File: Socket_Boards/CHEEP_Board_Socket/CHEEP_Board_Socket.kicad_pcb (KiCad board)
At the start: 4 copper layers, 64.9 x 71.4 mm, 70 parts

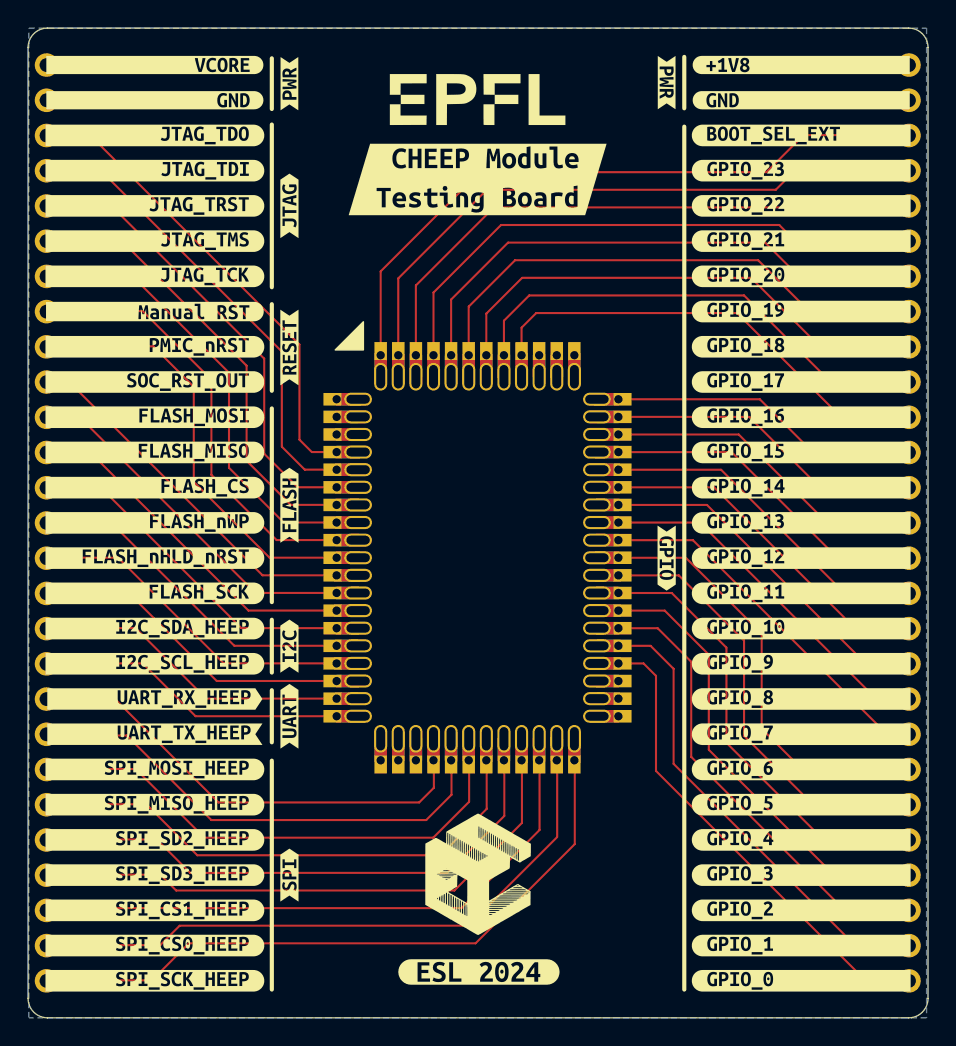
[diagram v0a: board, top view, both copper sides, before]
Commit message: Big push. Fixed the issues that were pending. See github
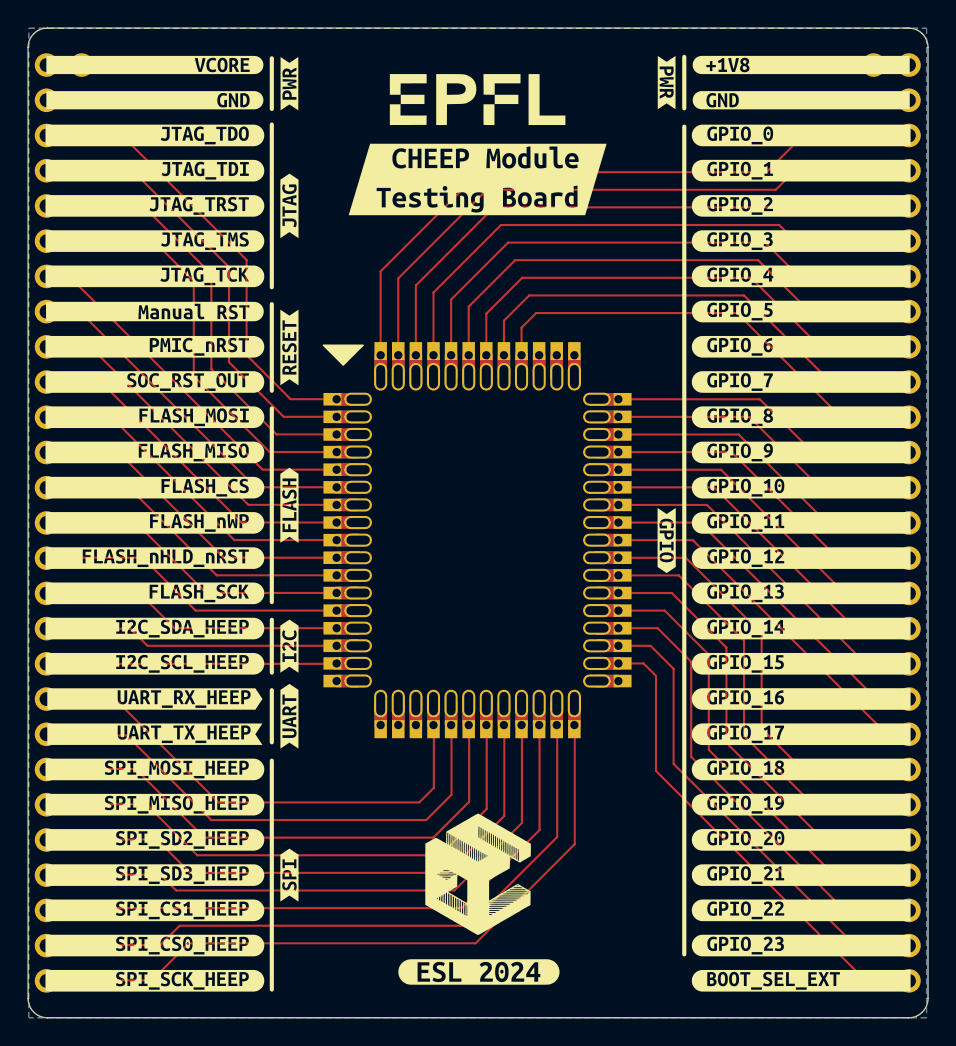
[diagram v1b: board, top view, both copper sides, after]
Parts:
- moved kibuzzard-66E70DDA 61.0 mm to (165.7, 135.3)
- moved kibuzzard-66E70EAB 61.0 mm to (165.7, 74.3)
- moved kibuzzard-66E70E24 55.9 mm to (165.7, 132.7)
- moved kibuzzard-66E70EA7 55.9 mm to (165.7, 76.8)
- moved kibuzzard-66E70E1C 50.8 mm to (165.7, 130.2)
- moved kibuzzard-66E70E9D 50.8 mm to (165.7, 79.4)
- moved kibuzzard-66E70E2E 45.7 mm to (165.7, 127.6)
- moved kibuzzard-66E70E98 45.7 mm to (165.7, 81.9)
- moved kibuzzard-66E70E32 40.6 mm to (165.7, 125.1)
- moved kibuzzard-66E70E93 40.6 mm to (165.7, 84.5)
- moved kibuzzard-66E70E38 35.6 mm to (165.7, 122.6)
- moved kibuzzard-66E70E8D 35.6 mm to (165.7, 87.0)
- moved kibuzzard-66E70E42 30.5 mm to (165.7, 120.0)
- moved kibuzzard-66E70E85 30.5 mm to (165.7, 89.5)
- moved kibuzzard-66E70E46 25.4 mm to (165.7, 117.5)
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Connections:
- J1 pad 1: VCORE -> Net-(J1A-JTAG_TDO)
- J1 pad 10: Net-(J1A-PMIC_nRST) -> Net-(J1A-FLASH_MISO)
- J1 pad 11: Net-(J1A-SOC_RST_OUT) -> Net-(J1A-FLASH_CS)
- J1 pad 12: Net-(J1A-FLASH_MOSI) -> Net-(J1A-FLASH_nWP)
- J1 pad 13: Net-(J1A-FLASH_MISO) -> Net-(J1A-FLASH_nHLD_nRST)
- J1 pad 14: Net-(J1A-FLASH_CS) -> Net-(J1A-FLASH_SCK)
- J1 pad 15: Net-(J1A-FLASH_nWP) -> Net-(J1A-I2C_SDA_HEEP)
- J1 pad 16: Net-(J1A-FLASH_nHLD_nRST) -> Net-(J1A-I2C_SCL_HEEP)
- J1 pad 17: Net-(J1A-FLASH_SCK) -> GND
- J1 pad 18: Net-(J1A-I2C_SDA_HEEP) -> +1V8
- J1 pad 19: Net-(J1A-I2C_SCL_HEEP) -> VCORE
- J1 pad 2: +1V8 -> Net-(J1A-JTAG_TDI)
- J1 pad 20: +1V8 -> GND
- J1 pad 21: VCORE -> Net-(J1B-UART_RX_HEEP)
- J1 pad 22: GND -> Net-(J1B-UART_TX_HEEP)
- J1 pad 23: Net-(J1B-UART_RX_HEEP) -> Net-(J1B-SPI_MOSI_HEEP)
- J1 pad 24: Net-(J1B-UART_TX_HEEP) -> Net-(J1B-SPI_MISO_HEEP)
- J1 pad 25: Net-(J1B-SPI_MOSI_HEEP) -> Net-(J1B-SPI_SD2_HEEP)
- J1 pad 26: Net-(J1B-SPI_MISO_HEEP) -> Net-(J1B-SPI_SD3_HEEP)
- J1 pad 27: Net-(J1B-SPI_SD2_HEEP) -> Net-(J1B-SPI_CS1_HEEP)
- J1 pad 28: Net-(J1B-SPI_SD3_HEEP) -> Net-(J1B-SPI_CS0_HEEP)
- J1 pad 29: Net-(J1B-SPI_CS1_HEEP) -> Net-(J1B-SPI_SCK_HEEP)
- J1 pad 3: GND -> Net-(J1A-JTAG_TRST)
- J1 pad 30: Net-(J1B-SPI_CS0_HEEP) -> GND
- J1 pad 31: Net-(J1B-SPI_SCK_HEEP) -> Net-(J1C-BOOT_SEL_EXT)
- J1 pad 32: +1V8 -> Net-(J1C-GPIO_23)
- J1 pad 33: VCORE -> Net-(J1C-GPIO_22)
- J1 pad 34: GND -> Net-(J1C-GPIO_21)
- J1 pad 35: Net-(J1C-BOOT_SEL_EXT) -> Net-(J1C-GPIO_20)
- J1 pad 36: Net-(J1C-GPIO_23) -> Net-(J1C-GPIO_19)
- J1 pad 37: Net-(J1C-GPIO_22) -> Net-(J1C-GPIO_18)
- J1 pad 38: Net-(J1C-GPIO_21) -> Net-(J1C-GPIO_17)
- J1 pad 39: Net-(J1C-GPIO_20) -> Net-(J1C-GPIO_16)
- J1 pad 4: Net-(J1A-JTAG_TDO) -> Net-(J1A-JTAG_TMS)
- J1 pad 40: Net-(J1C-GPIO_19) -> Net-(J1C-GPIO_15)
- J1 pad 41: Net-(J1C-GPIO_18) -> Net-(J1C-GPIO_14)
- J1 pad 42: Net-(J1C-GPIO_17) -> Net-(J1C-GPIO_13)
- J1 pad 43: Net-(J1C-GPIO_16) -> Net-(J1C-GPIO_12)
- J1 pad 44: Net-(J1C-GPIO_15) -> Net-(J1C-GPIO_11)
- J1 pad 45: Net-(J1C-GPIO_14) -> Net-(J1C-GPIO_10)
- J1 pad 46: Net-(J1C-GPIO_13) -> Net-(J1C-GPIO_9)
- J1 pad 47: Net-(J1C-GPIO_12) -> VCORE
- J1 pad 48: Net-(J1C-GPIO_11) -> +1V8
- J1 pad 49: Net-(J1C-GPIO_10) -> GND
- J1 pad 5: Net-(J1A-JTAG_TDI) -> Net-(J1A-JTAG_TCK)
- J1 pad 50: Net-(J1C-GPIO_9) -> Net-(J1D-GPIO_8)
- J1 pad 51: VCORE -> Net-(J1D-GPIO_7)
- J1 pad 52: +1V8 -> Net-(J1D-GPIO_6)
- J1 pad 53: GND -> Net-(J1D-GPIO_5)
- J1 pad 54: Net-(J1D-GPIO_8) -> Net-(J1D-GPIO_4)
- J1 pad 55: Net-(J1D-GPIO_7) -> Net-(J1D-GPIO_3)
- J1 pad 56: Net-(J1D-GPIO_6) -> Net-(J1D-GPIO_2)
- J1 pad 57: Net-(J1D-GPIO_5) -> Net-(J1D-GPIO_1)
- J1 pad 58: Net-(J1D-GPIO_4) -> Net-(J1D-GPIO_0)
- J1 pad 6: Net-(J1A-JTAG_TRST) -> Net-(J1A-Manual_RST)
- J1 pad 7: Net-(J1A-JTAG_TMS) -> Net-(J1A-PMIC_nRST)
- J1 pad 8: Net-(J1A-JTAG_TCK) -> Net-(J1A-SOC_RST_OUT)
- J1 pad 9: Net-(J1A-Manual_RST) -> Net-(J1A-FLASH_MOSI)
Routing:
- net VCORE: track 24.8 -> 12.4 mm
- net +1V8: track 24.8 -> 12.4 mm
- net Net-(J1A-PMIC_nRST): track 36.7 -> 31.1 mm
- net Net-(J1A-Manual_RST): track 37.0 -> 31.4 mm
- net Net-(J1A-JTAG_TCK): track 37.5 -> 31.9 mm
- net Net-(J1B-SPI_MISO_HEEP): track 43.6 -> 46.1 mm
- net Net-(J1B-UART_RX_HEEP): track 38.9 -> 41.4 mm
- net Net-(J1B-SPI_SD3_HEEP): track 46.7 -> 49.2 mm
- net Net-(J1B-SPI_SCK_HEEP): track 53.6 -> 56.2 mm
- net Net-(J1B-SPI_MOSI_HEEP): track 42.0 -> 44.5 mm
- net Net-(J1B-SPI_CS1_HEEP): track 48.4 -> 50.9 mm
- net Net-(J1B-UART_TX_HEEP): track 40.4 -> 43.0 mm
- net Net-(J1B-SPI_SD2_HEEP): track 45.1 -> 47.7 mm
- net Net-(J1B-SPI_CS0_HEEP): track 51.0 -> 53.5 mm
- net Net-(J1A-JTAG_TDI): track 39.1 -> 37.5 mm
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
